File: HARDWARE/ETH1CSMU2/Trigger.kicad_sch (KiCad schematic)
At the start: 22 parts, among them U701 TXB0104PW, U702 ADuM5402, U703 74AC125

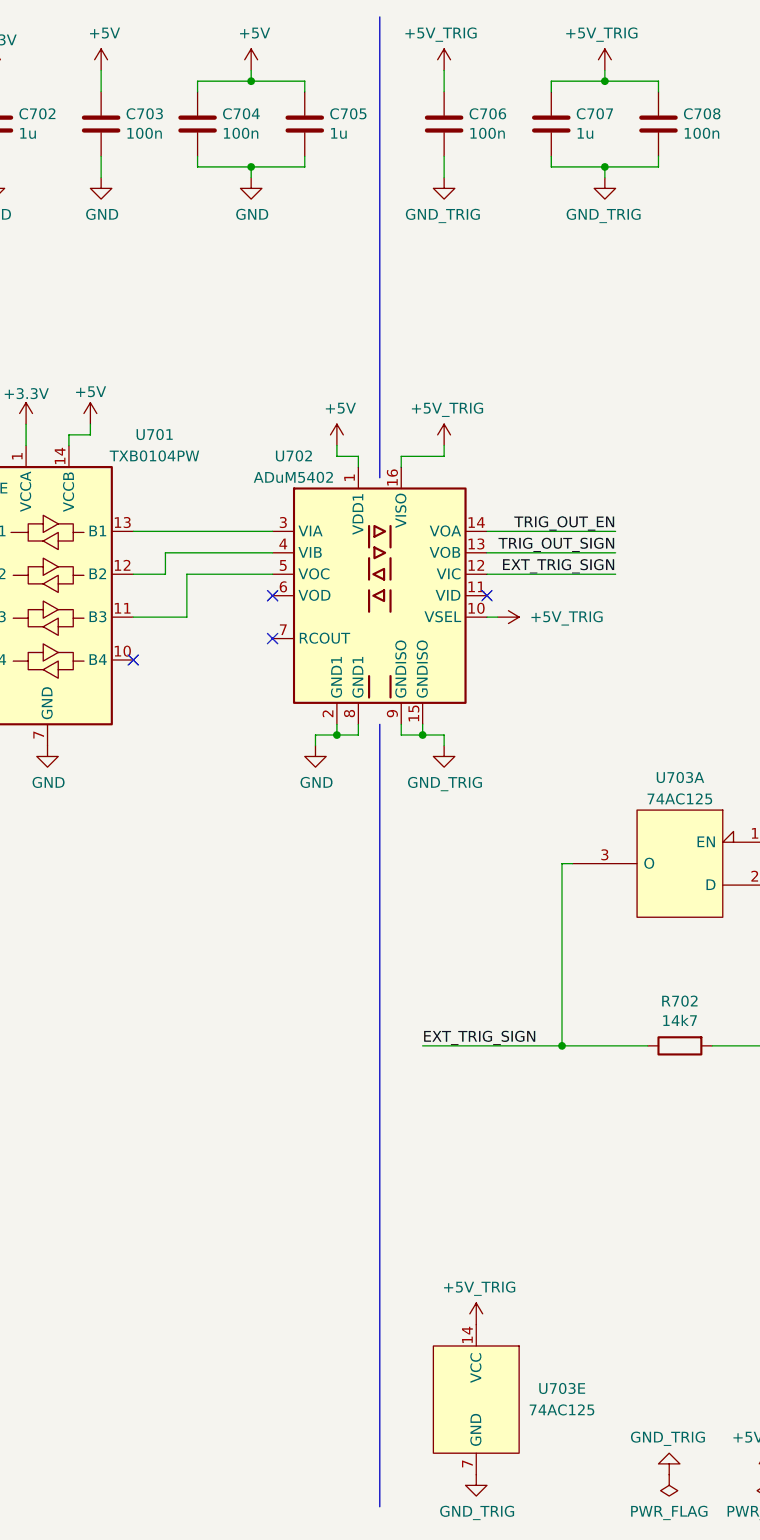
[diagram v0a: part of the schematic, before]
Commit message: Development
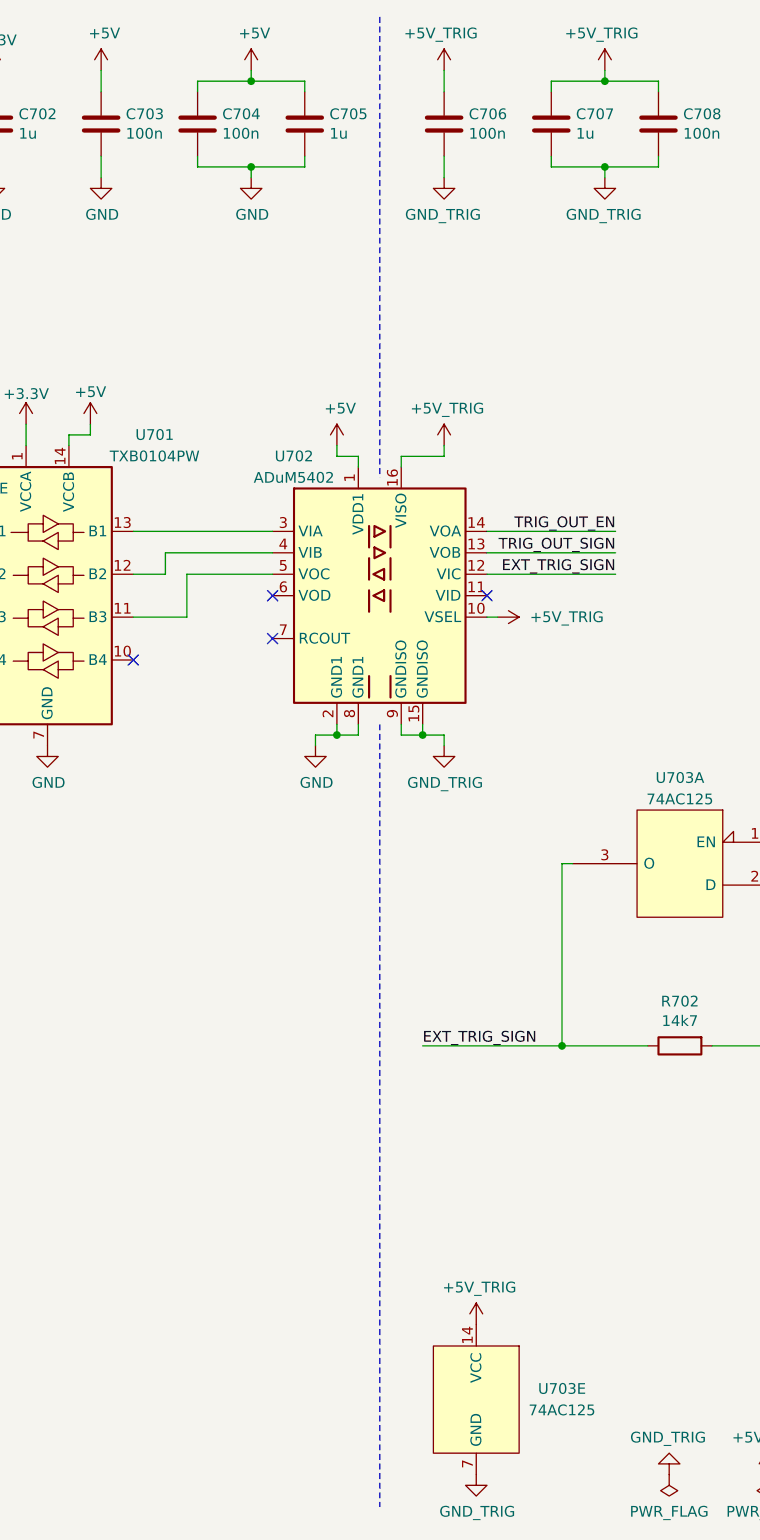
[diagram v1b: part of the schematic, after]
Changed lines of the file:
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@@
   )
   (polyline (pts (xy 115.57 99.06) (xy 115.57 191.77))
-    (stroke (width 0) (type default))
+    (stroke (width 0) (type dash))
   )
   (wire (pts (xy 137.16 115.57) (xy 138.43 115.57))
@@
   )
   (polyline (pts (xy 115.57 15.24) (xy 115.57 69.85))
-    (stroke (width 0) (type default))
+    (stroke (width 0) (type dash))
   )
   (wire (pts (xy 102.87 78.74) (xy 90.17 78.74))
